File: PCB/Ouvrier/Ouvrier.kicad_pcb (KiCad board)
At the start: 2 copper layers, 52 x 54.5 mm, 17 parts, among them J1 Batterie, J2 VBAT Xiao, J3 DC 5V input, Q1 2N2222B, U1 XIAO-ESP32-S3-Plus-DIP, U2 BMP581, U3 UWB

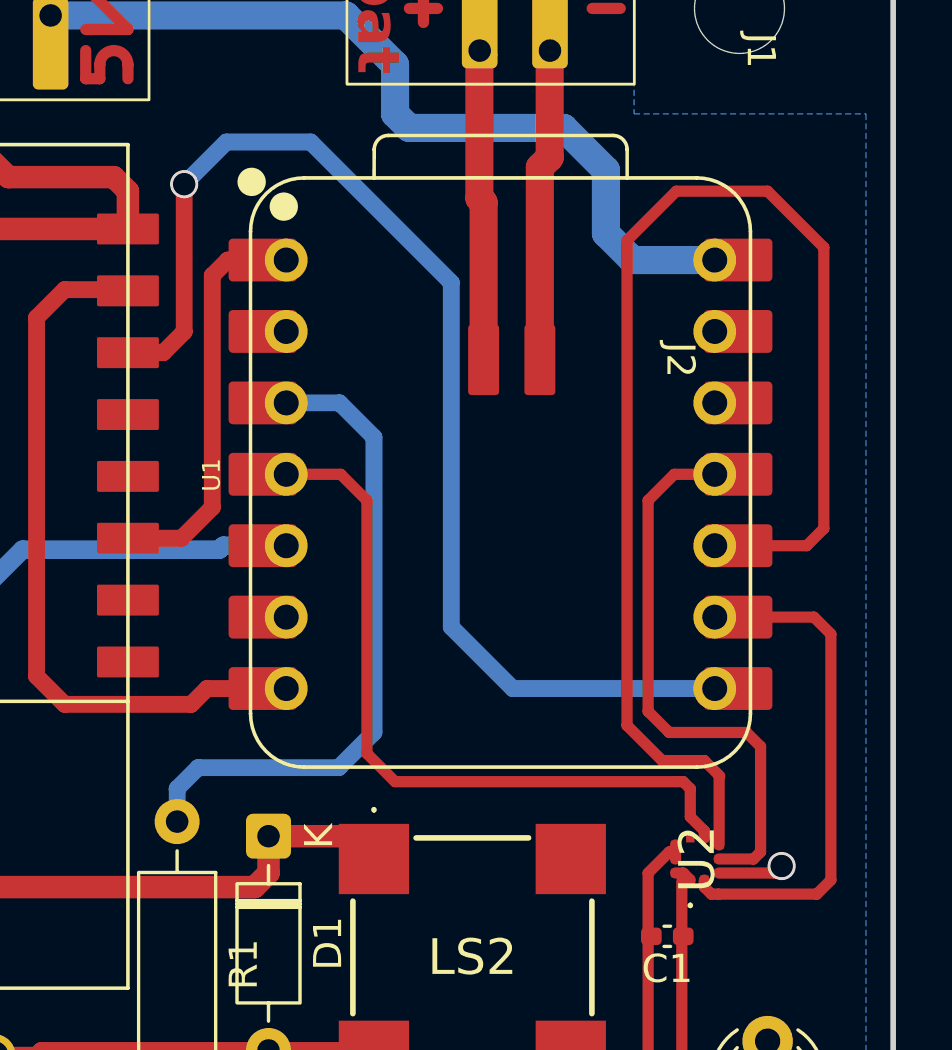
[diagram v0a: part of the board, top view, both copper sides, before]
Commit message: gbr
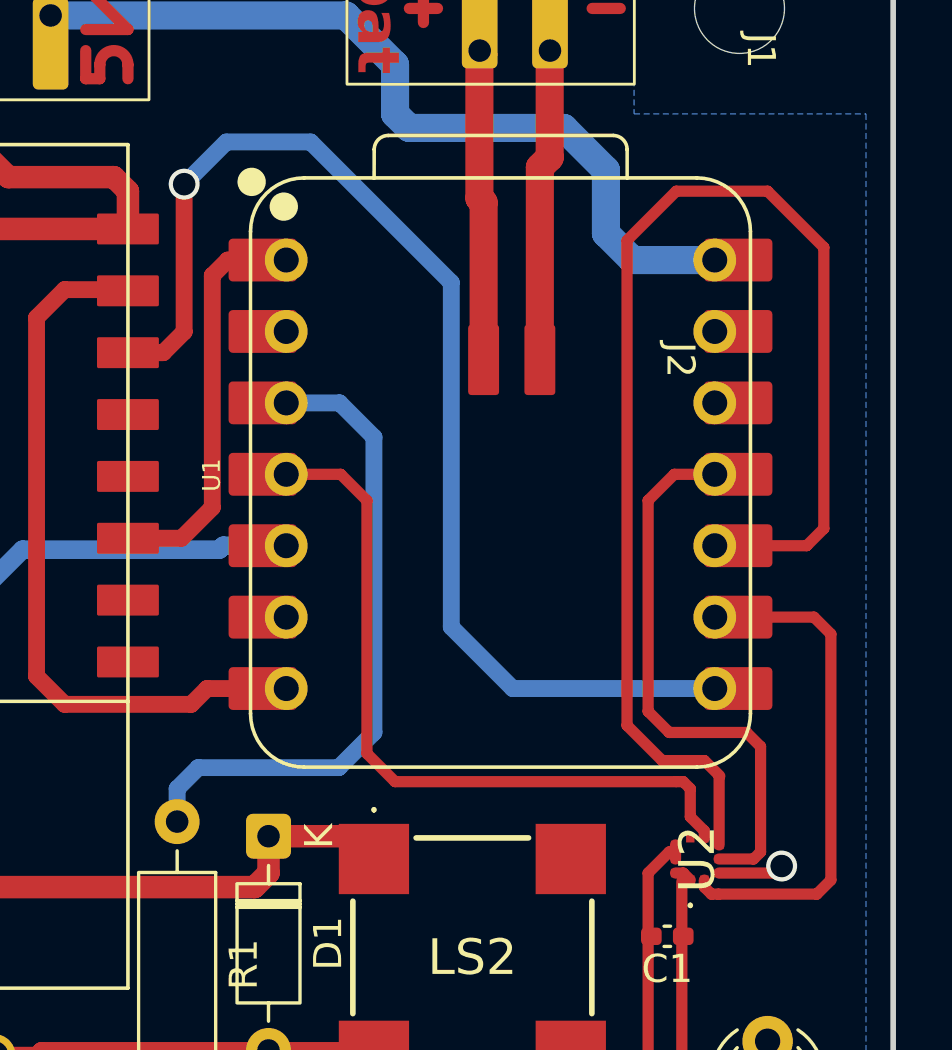
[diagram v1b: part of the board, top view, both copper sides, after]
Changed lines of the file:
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@@
 		(filling no)
 		(pcbplotparams
-			(layerselection 0x00000000_00000000_55555555_5755f5ff)
-			(plot_on_all_layers_selection 0x00000000_00000000_00000000_00000000)
+			(layerselection 0x00000000_00000000_55555555_57555555)
+			(plot_on_all_layers_selection 0x00000000_00000000_00000000_02000000)
 			(disableapertmacros no)
 			(usegerberextensions no)
@@
 			(outputformat 1)
 			(mirror no)
-			(drillshape 1)
+			(drillshape 0)
 			(scaleselection 1)
 			(outputdirectory "")
@@
 	(via
 		(at 141.5 90.5)
-		(size 1)
+		(size 1.1)
 		(drill 0.8)
 		(layers "F.Cu" "B.Cu")
@@
 	(via
 		(at 120.25 66.25)
-		(size 1)
+		(size 1.1)
 		(drill 0.8)
 		(layers "F.Cu" "B.Cu")
